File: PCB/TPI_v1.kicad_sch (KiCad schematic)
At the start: 7 parts, among them J1 Raspberry pi zero w, J2 BME280, J3 BME280, J4 MQ135, U1 BMI160, U2 DS18B20

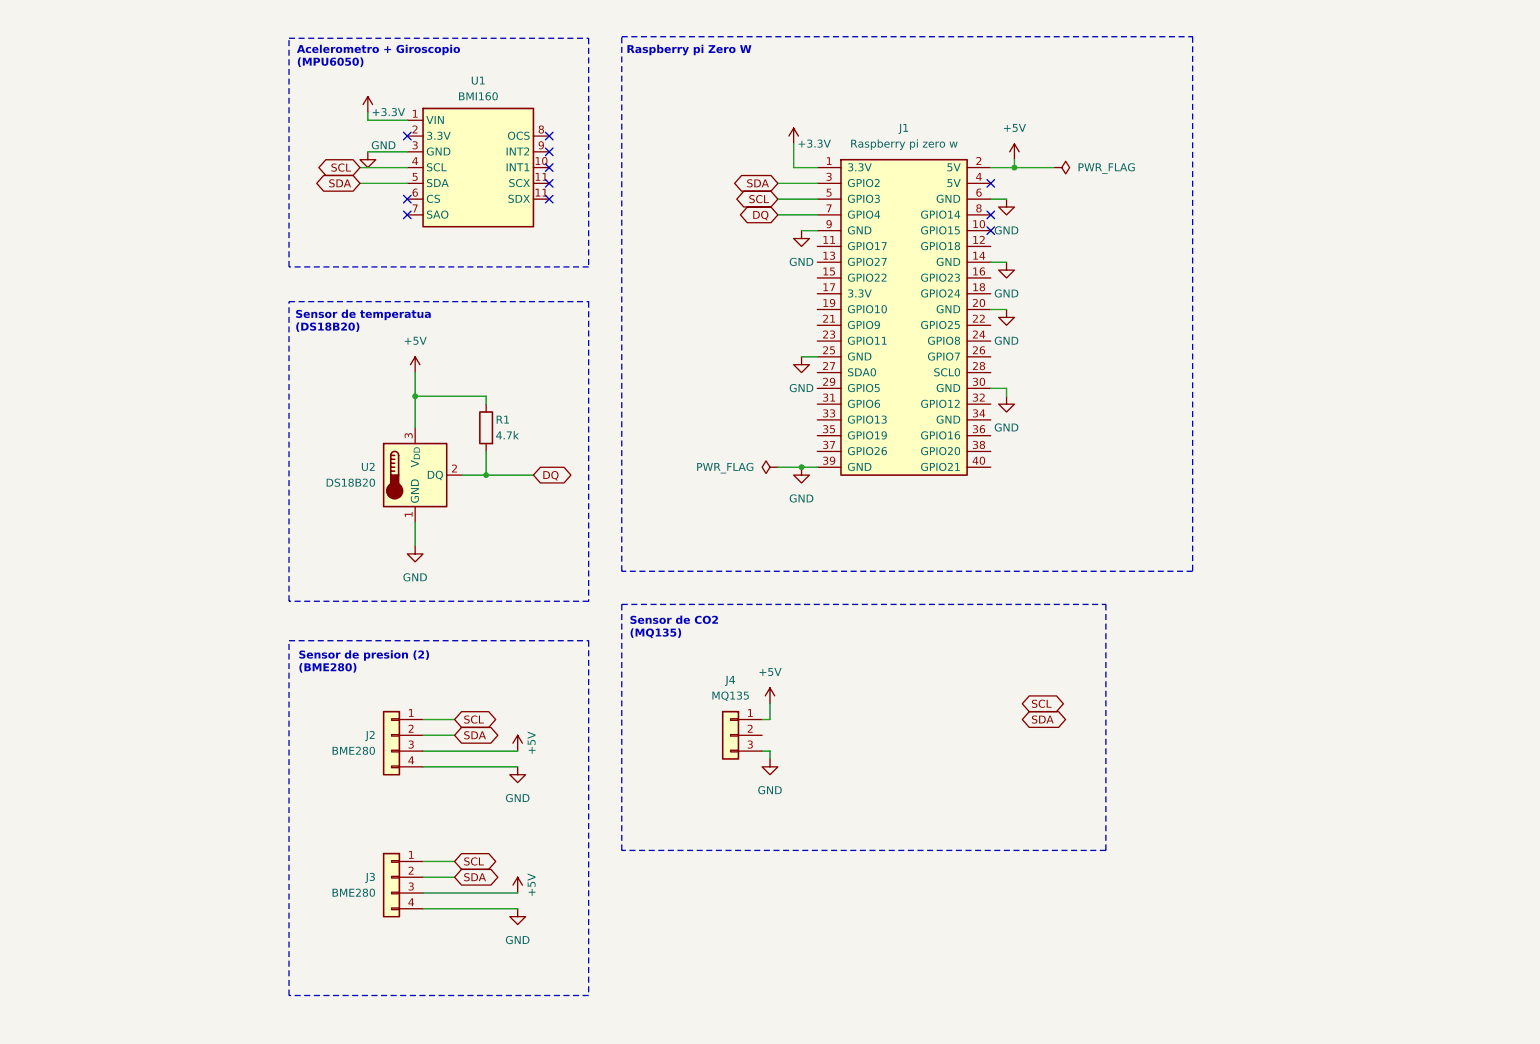
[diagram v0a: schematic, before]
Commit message: PCB update
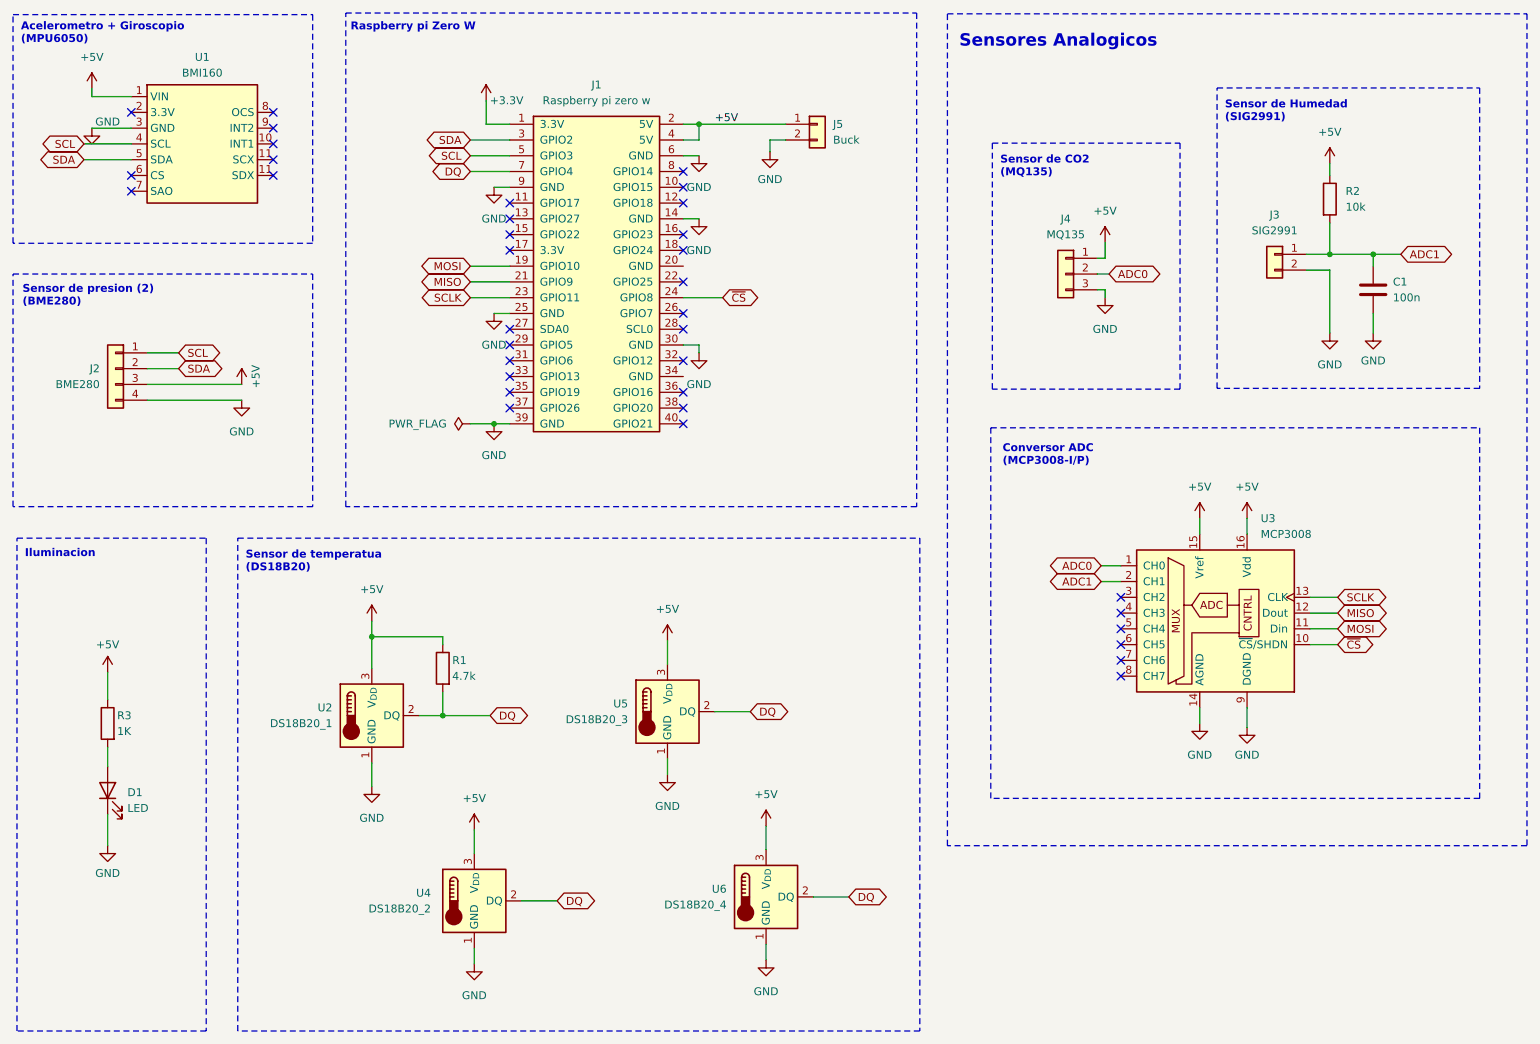
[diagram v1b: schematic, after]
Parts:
- removed J3: BME280, Connector_JST:JST_PH_S4B-PH-K_1x04_P2.00mm_Horizontal, symbol Connector_Generic:Conn_01x04
- added C1: 100n, Capacitor_THT:C_Disc_D3.0mm_W1.6mm_P2.50mm, symbol Device:C
- added D1: LED, symbol Device:LED
- added J3: SIG2991, Connector_JST:JST_XH_S2B-XH-A-1_1x02_P2.50mm_Horizontal, symbol Connector_Generic:Conn_01x02
- added J5: Buck, Connector_PinSocket_2.54mm:PinSocket_2x01_P2.54mm_Vertical, symbol Connector_Generic:Conn_01x02
- added R2: 10k, Resistor_THT:R_Axial_DIN0207_L6.3mm_D2.5mm_P7.62mm_Horizontal, symbol Device:R
- added R3: 1K, Resistor_THT:R_Axial_DIN0207_L6.3mm_D2.5mm_P7.62mm_Horizontal, symbol Device:R
- added U3: MCP3008, Package_DIP:DIP-16_W7.62mm, symbol Analog_ADC:MCP3008
- added U4: DS18B20_2, Connector_JST:JST_XH_S3B-XH-A-1_1x03_P2.50mm_Horizontal, symbol Sensor_Temperature:DS18B20
- added U5: DS18B20_3, Connector_JST:JST_XH_S3B-XH-A-1_1x03_P2.50mm_Horizontal, symbol Sensor_Temperature:DS18B20
- added U6: DS18B20_4, Connector_JST:JST_XH_S3B-XH-A-1_1x03_P2.50mm_Horizontal, symbol Sensor_Temperature:DS18B20
- J2: footprint Connector_JST:JST_PH_S4B-PH-K_1x04_P2.00mm_Horizontal -> Connector_JST:JST_XH_S4B-XH-A-1_1x04_P2.50mm_Horizontal
- J4: footprint (none) -> Connector_JST:JST_XH_B3B-XH-A_1x03_P2.50mm_Vertical
- U2: value DS18B20 -> DS18B20_1; footprint Connector_JST:JST_PH_S3B-PH-K_1x03_P2.00mm_Horizontal -> Connector_JST:JST_XH_S3B-XH-A-1_1x03_P2.50mm_Horizontal
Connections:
- net +3.3V: no longer U1.1 (VIN)
- net +5V: now also J1.4 (5V), U1.1 (VIN), J5.1 (Pin_1), R2.1, R3.1, U3.15 (Vref), U3.16 (Vdd), U4.3 (V_{DD}), U5.3 (V_{DD}), U6.3 (V_{DD})
- net DQ: now also U4.2 (DQ), U5.2 (DQ), U6.2 (DQ)
- net GND: now also C1.2, D1.1 (K), J3.2 (Pin_2), J5.2 (Pin_2), U3.14 (AGND), U3.9 (DGND), U4.1 (GND), U5.1 (GND), U6.1 (GND); no longer J1.20 (GND)
- net ADC0: now reaches J4.2 (Pin_2)
- net ADC0: now also U3.1 (CH0)
- net MOSI: now reaches J1.19 (GPIO10)
- net MOSI: now also U3.11 (Din)
- net MISO: now reaches J1.21 (GPIO9)
- net MISO: now also U3.12 (Dout)
- net SCLK: now reaches J1.23 (GPIO11)
- net SCLK: now also U3.13 (CLK)
- net ~{CS}: now reaches J1.24 (GPIO8)
- net ~{CS}: now also U3.10 (~{CS}/SHDN)
- new net: D1.2 (A), R3.2
- new net ADC1: C1.1, J3.1 (Pin_1), R2.2, U3.2 (CH1)
- no-connect marks 11 -> 36
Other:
- note added: "Conversor ADC (MCP3008-I/P)"
- note added: "Iluminacion"
- note added: "Sensor de Humedad (SIG2991)"
- note added: "Sensores Analogicos"
- title: (none) -> WALL-E Hat
- moved on the sheet: J1, J2, J4, R1, U1, U2
